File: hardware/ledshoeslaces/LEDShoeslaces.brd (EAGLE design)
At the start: 50 x 38 mm, 13 parts, among them IC1 LM1117MPX-5.0

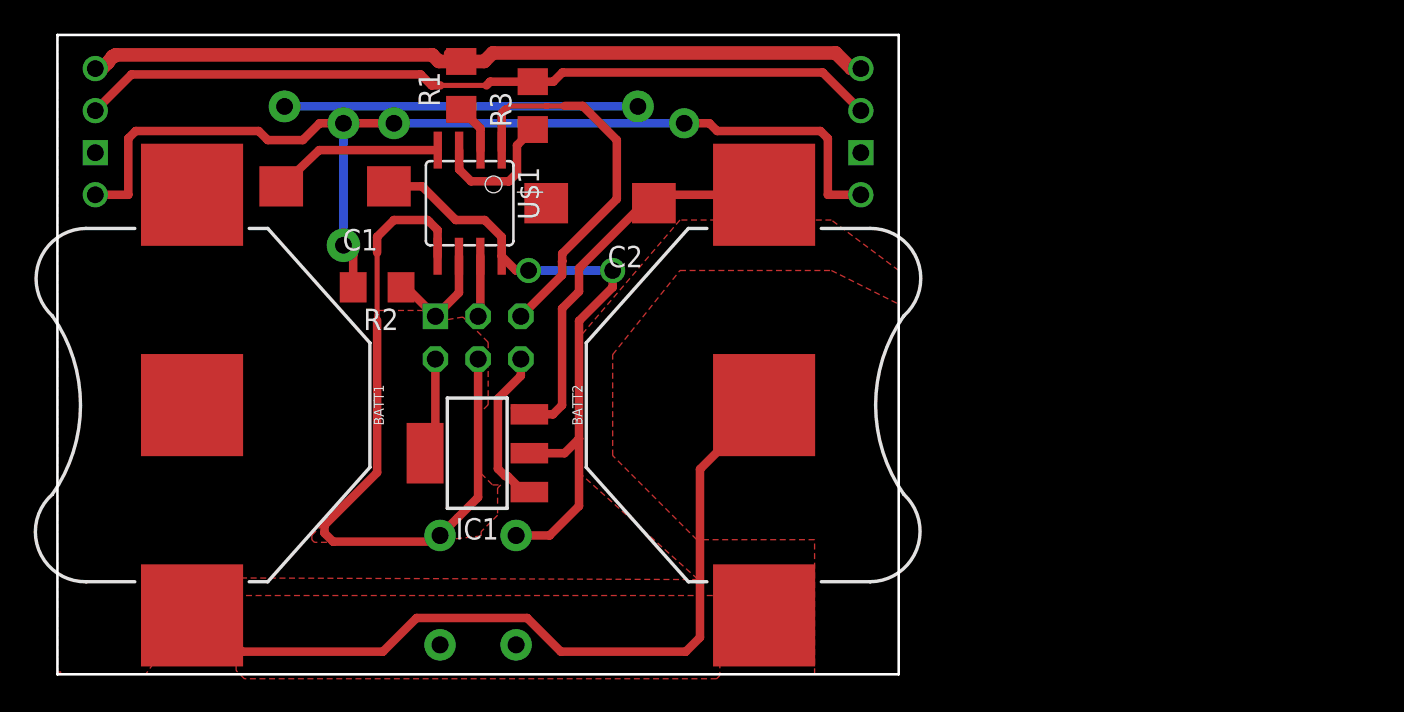
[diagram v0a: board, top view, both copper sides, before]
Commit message: zzZZzZZZzzz
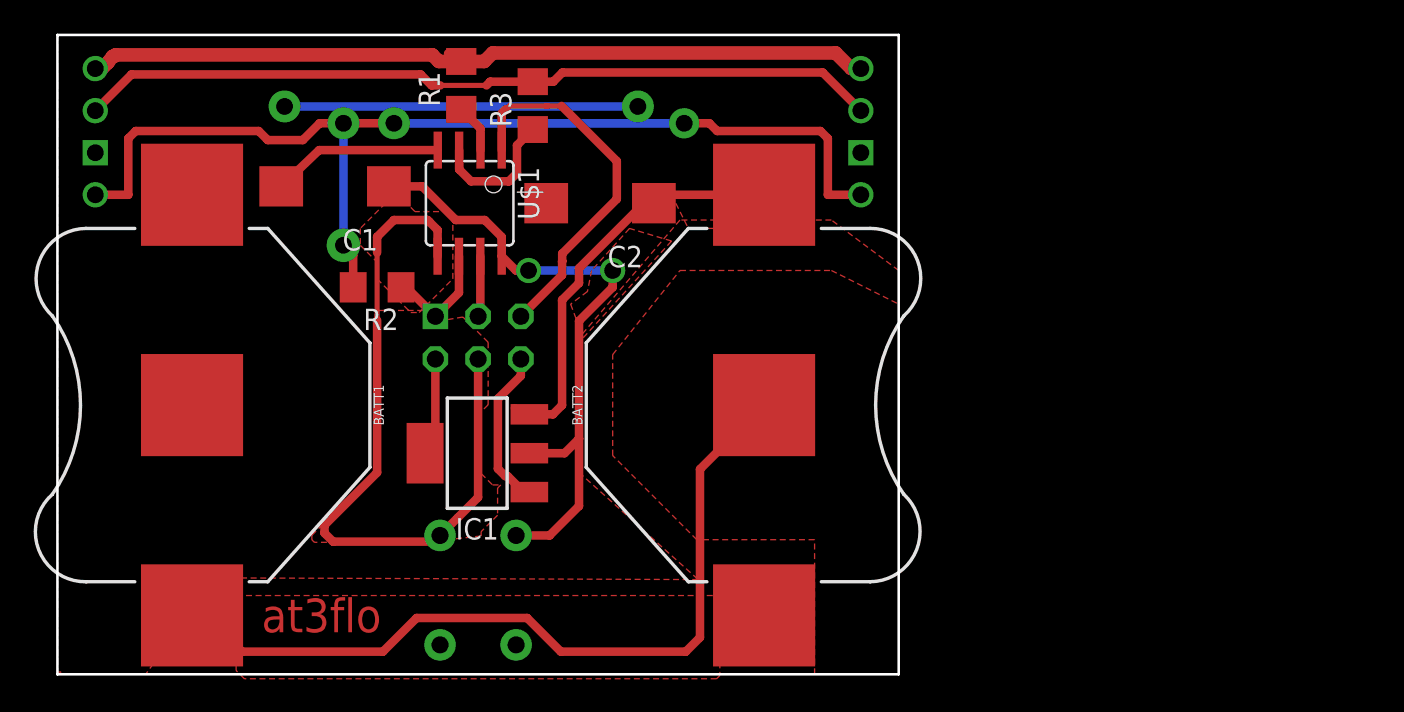
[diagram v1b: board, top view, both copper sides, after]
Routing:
- net RST: track 23.3 -> 22.6 mm
- added copper zone on layer 1, net MOSI
- added copper zone on layer 1, net V_BATT
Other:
- board text added: "numerik games 2017"
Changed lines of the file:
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@@
 <rectangle x1="0.183940625" y1="0.178859375" x2="0.18859375" y2="0.17928125" layer="1"/>
 <text x="0" y="-0.002115625" size="0.000846875" layer="1" font="vector">/ws/ng2017/assets/img/logo-600x600.bmp</text>
-<text x="13" y="3.75" size="0.000846875" layer="1" font="vector">at3flo</text>
+<text x="13.25" y="3.5" size="0.000846875" layer="1" font="vector">at3flo</text>
+<text x="19.25" y="4.5" size="2" layer="1" font="vector" rot="R180">at3flo</text>
+<text x="78" y="14.25" size="0.000846875" layer="1" font="vector">numerik games 2017</text>
 </plain>
 <attributes>
@@
 <wire x1="28" y1="24" x2="27.2513" y2="24" width="0.508" layer="1"/>
 <wire x1="27.2513" y1="24" x2="26.405" y2="24.8463" width="0.508" layer="1"/>
-<wire x1="28.049" y1="13.14" x2="30.14" y2="13.14" width="0.508" layer="1"/>
-<wire x1="31" y1="14" x2="30.14" y2="13.14" width="0.508" layer="1"/>
 <wire x1="31" y1="14" x2="31" y2="21" width="0.508" layer="1"/>
 <wire x1="27.2606" y1="8.2512" x2="29.2512" y2="8.2512" width="0.508" layer="1"/>
@@
 <wire x1="26.405" y1="24.8463" x2="26.405" y2="25.99261875" width="0.508" layer="1"/>
 <wire x1="26.405" y1="25.99261875" x2="25.39761875" y2="27" width="0.508" layer="1"/>
+<polygon width="0.508" layer="1">
+<vertex x="31.75" y="24"/>
+<vertex x="31.5" y="22.75"/>
+<vertex x="30.5" y="22"/>
+<vertex x="31.25" y="20"/>
+<vertex x="36.5" y="25.75"/>
+<vertex x="34" y="26.5"/>
+</polygon>
+<wire x1="28.049" y1="13.14" x2="30.14" y2="13.14" width="0.508" layer="1"/>
+<wire x1="30.14" y1="13.14" x2="31" y2="14" width="0.508" layer="1"/>
 <wire x1="22.46188125" y1="13.75088125" x2="28.049" y2="13.14" width="0" layer="19" extent="1-1"/>
 </signal>
@@
 <wire x1="25.00188125" y1="18.736903125" x2="25.00188125" y2="10.516296875" width="0.508" layer="1"/>
 <wire x1="19" y1="21.04174375" x2="19" y2="25.0575625" width="0.3048" layer="1"/>
+<polygon width="0.508" layer="1">
+<vertex x="20.75" y="28"/>
+<vertex x="19.5" y="28"/>
+<vertex x="18" y="26.5"/>
+<vertex x="18" y="25.5"/>
+<vertex x="19" y="24.5"/>
+<vertex x="19" y="23.5"/>
+<vertex x="21" y="21.5"/>
+<vertex x="21.5" y="21.5"/>
+<vertex x="23.5" y="23.5"/>
+<vertex x="23.5" y="27.25"/>
+<vertex x="23.25" y="27.5"/>
+<vertex x="21.25" y="27.5"/>
+</polygon>
 </signal>
 <signal name="MISO">
@@
 <wire x1="26.405" y1="31.1543" x2="26.405" y2="33.33755625" width="0.508" layer="1"/>
 <wire x1="26.6620375" y1="33.59459375" x2="26.405" y2="33.33755625" width="0.508" layer="1"/>
-<wire x1="30.151871875" y1="33.7812" x2="31.2188" y2="33.7812" width="0.508" layer="1"/>
-<wire x1="31.2188" y1="33.7812" x2="33.246" y2="31.754" width="0.508" layer="1"/>
-<wire x1="33.246" y1="28.246" x2="30" y2="25" width="0.508" layer="1"/>
+<wire x1="30" y1="25" x2="33.246" y2="28.246" width="0.508" layer="1"/>
 <wire x1="30" y1="25" x2="30" y2="24.559128125" width="0.508" layer="1"/>
 <wire x1="30" y1="24.559128125" x2="29.99199375" y2="24.551121875" width="0.508" layer="1"/>
 <wire x1="29.99199375" y1="24.551121875" x2="29.99199375" y2="23.727015625" width="0.508" layer="1"/>
 <wire x1="29.99199375" y1="23.727015625" x2="27.54188125" y2="21.276903125" width="0.508" layer="1"/>
-<wire x1="33.246" y1="31.754" x2="33.246" y2="28.246" width="0.508" layer="1"/>
 <wire x1="29.15135625" y1="33.7812" x2="29" y2="33.7812" width="0.3048" layer="1"/>
-<wire x1="29.15135625" y1="33.7812" x2="30.151871875" y2="33.7812" width="0.3048" layer="1"/>
+<wire x1="29.965021875" y1="33.7812" x2="29.15135625" y2="33.7812" width="0.3048" layer="1"/>
 <wire x1="29" y1="33.7812" x2="29.15135625" y2="33.7812" width="0.3048" layer="1"/>
 <wire x1="26.84864375" y1="33.7812" x2="26.6620375" y2="33.59459375" width="0.3048" layer="1"/>
 <wire x1="29" y1="33.7812" x2="26.84864375" y2="33.7812" width="0.3048" layer="1"/>
+<wire x1="33.246" y1="28.246" x2="33.246" y2="30.500221875" width="0.508" layer="1"/>
+<wire x1="33.246" y1="30.500221875" x2="29.965021875" y2="33.7812" width="0.508" layer="1"/>
 </signal>
 <signal name="BATS">
@@
 <wire x1="28.049" y1="15.451" x2="29.451" y2="15.451" width="0.508" layer="1"/>
 <wire x1="29.451" y1="15.451" x2="29.992" y2="15.992" width="0.508" layer="1"/>
-<wire x1="29.992" y1="21.738121875" x2="29.992" y2="15.992" width="0.508" layer="1"/>
-<wire x1="29.992" y1="21.738121875" x2="31" y2="22.746121875" width="0.508" layer="1"/>
-<wire x1="31" y1="24.1335875" x2="31" y2="22.746121875" width="0.508" layer="1"/>
+<wire x1="31" y1="23.253325" x2="31" y2="24.1335875" width="0.508" layer="1"/>
+<wire x1="29.992" y1="22.245325" x2="31" y2="23.253325" width="0.508" layer="1"/>
+<wire x1="29.992" y1="15.992" x2="29.992" y2="22.245325" width="0.508" layer="1"/>
+<polygon width="0.508" layer="1">
+<vertex x="36.5" y="28.5"/>
+<vertex x="37.5" y="26.5"/>
+<vertex x="39.5" y="26.5"/>
+<vertex x="39.75" y="28.25"/>
+</polygon>
 </signal>
 <signal name="LEDRED">
